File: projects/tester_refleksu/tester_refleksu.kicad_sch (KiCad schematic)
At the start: 25 parts, among them J1 +, J2 −, SW1 SW_Push_4P, SW2 SW_Push_4P, T1 BC548, T2 BC548, T3 BC557

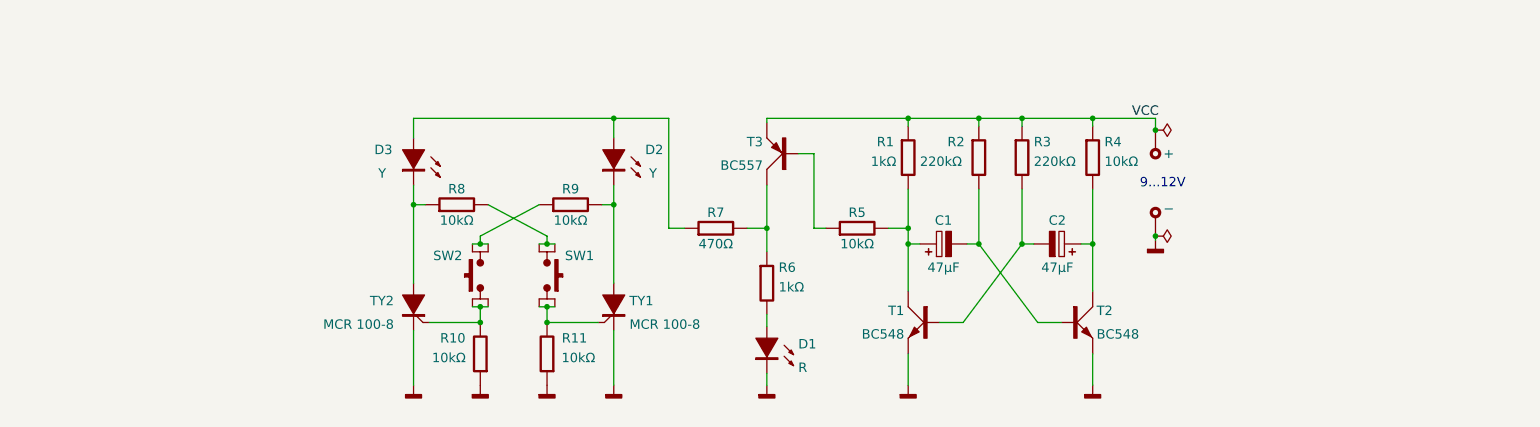
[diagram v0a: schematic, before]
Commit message: tester_refleksu_r2
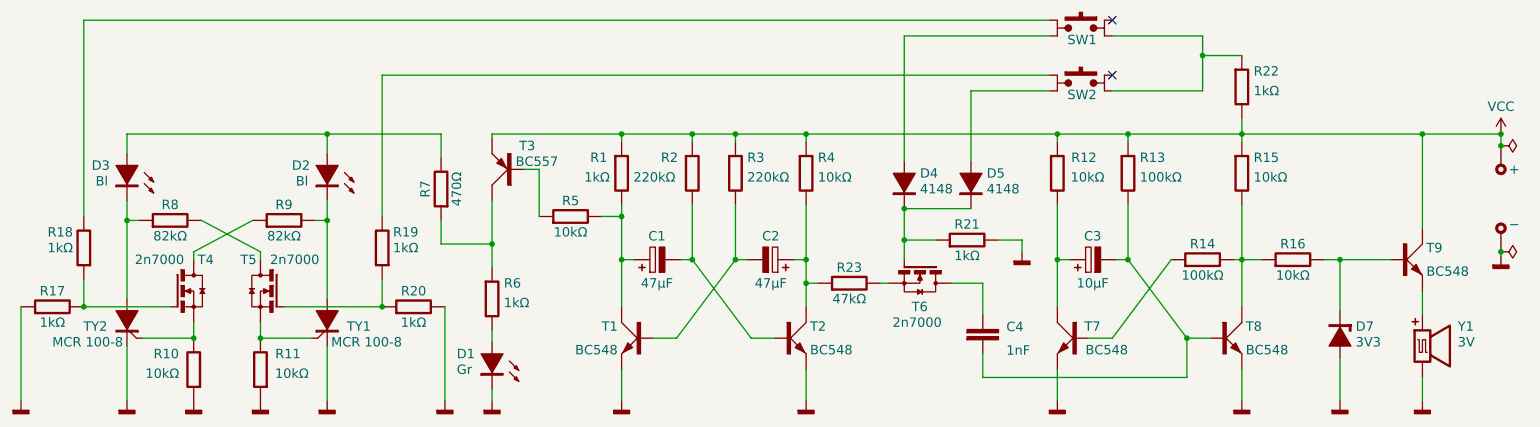
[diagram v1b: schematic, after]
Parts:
- added C3: 10μF, VeeCad:RA1_2, symbol Custom_Generic:C_Polarized
- added C4: 1nF, symbol *Custom_Generic:C
- added D4, D5: 4148, symbol *Custom_Generic:D
- added D7: 3V3, symbol *Custom_Generic:D_zener
- added R12, R15, R16: 10kΩ, VeeCad:AX3_1N, symbol Custom_Generic:R
- added R13, R14: 100kΩ, VeeCad:AX3_1N, symbol Custom_Generic:R
- added R17, R20, R21, R22: 1kΩ, VeeCad:AX3_1N, symbol Custom_Generic:R
- added R18, R19: 1kΩ, VeeCad:VERTAX_1N_180, symbol Custom_Generic:R
- added R23: 47kΩ, VeeCad:AX3_1N, symbol Custom_Generic:R
- added T4, T5, T6: 2n7000, symbol *Custom_Generic:NMOS_SGD
- added T7, T8, T9: BC548, VeeCad:TO92, symbol Custom_Generic:NPN_BJT_CBE
- added Y1: 3V, symbol *Custom_Generic:Buzzer_Magnetic_Active
- D1: value R -> Gr
- D2, D3: value Y -> Bl
- R8, R9: value 10kΩ -> 82kΩ
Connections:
- net GNDD: now also D7.2 (A), R17.1, R20.2, R21.2, T7.3 (E), T8.3 (E), Y1.2
- net VCC: now also R12.1, R13.1, R15.1, R22.2, T9.1 (C)
- net at D2.2 (A), D3.2 (A): now also R7.2; no longer R7.1
- net at R6.1, T3.1 (C): now also R7.1; no longer R7.2
- net at R10.2, TY2.2 (G): now also T4.1 (S); no longer SW2.1 (1A), SW2.3 (1B)
- net at R11.2, TY1.2 (G): now also T5.1 (S); no longer SW1.1 (1A), SW1.3 (1B)
- net at C2.2 (+), R4.2, T2.1 (C): now also R23.1
- new net: R23.2, T6.1 (S)
- new net: D4.1 (K), D5.1 (K), R21.1, T6.2 (G)
- new net: C4.2, T6.3 (D)
- new net: R19.2, SW2.1 (1A)
- new net: D5.2 (A), SW2.3 (1B)
- new net: R22.1, SW1.3 (1B), SW2.4 (2B)
- new net: D7.1 (K), R16.2, T9.2 (B)
- new net: T9.3 (E), Y1.1
- new net: R17.2, R18.1, T4.2 (G)
- new net: R9.1, T4.3 (D)
- new net: C3.1 (-), C4.1, R13.2, T8.2 (B)
- new net: R18.2, SW1.2 (2A)
- new net: D4.2 (A), SW1.4 (2B)
- new net: C3.2 (+), R12.2, T7.1 (C)
- new net: R14.2, R15.2, R16.1, T8.1 (C)
- new net: R8.2, T5.3 (D)
- new net: R14.1, T7.2 (B)
- new net: R19.1, R20.1, T5.2 (G)
- now unconnected: SW2.2 (2A)
- no-connect marks 0 -> 2
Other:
- note removed: "9...12V"
- moved on the sheet: C1, C2, D1, D2, D3, R1, R10, R11, R2, R3, R4, R5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
